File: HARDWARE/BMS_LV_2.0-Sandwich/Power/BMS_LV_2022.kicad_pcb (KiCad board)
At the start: 4 copper layers, 90 x 45 mm, 104 parts, among them J1 Conn_01x26, J11 Conn_01x07_Female, J2 AS214-97PN, J4 Battery+, J5 Battery-, Q1 BC846, Q10 BSS138, Q12 SIR5607DP-T1-RE3, Q13 SIR5607DP-T1-RE3, Q14 SIR5607DP-T1-RE3, Q15 SIR5607DP-T1-RE3, Q2 ZXMN3F30FHTA, Q3 ZXMN3F30FHTA, Q4 ZXMN3F30FHTA, Q5 ZXMN3F30FHTA, Q6 ZXMN3F30FHTA, Q7 ZXMN3F30FHTA, U5 ACHS-7123

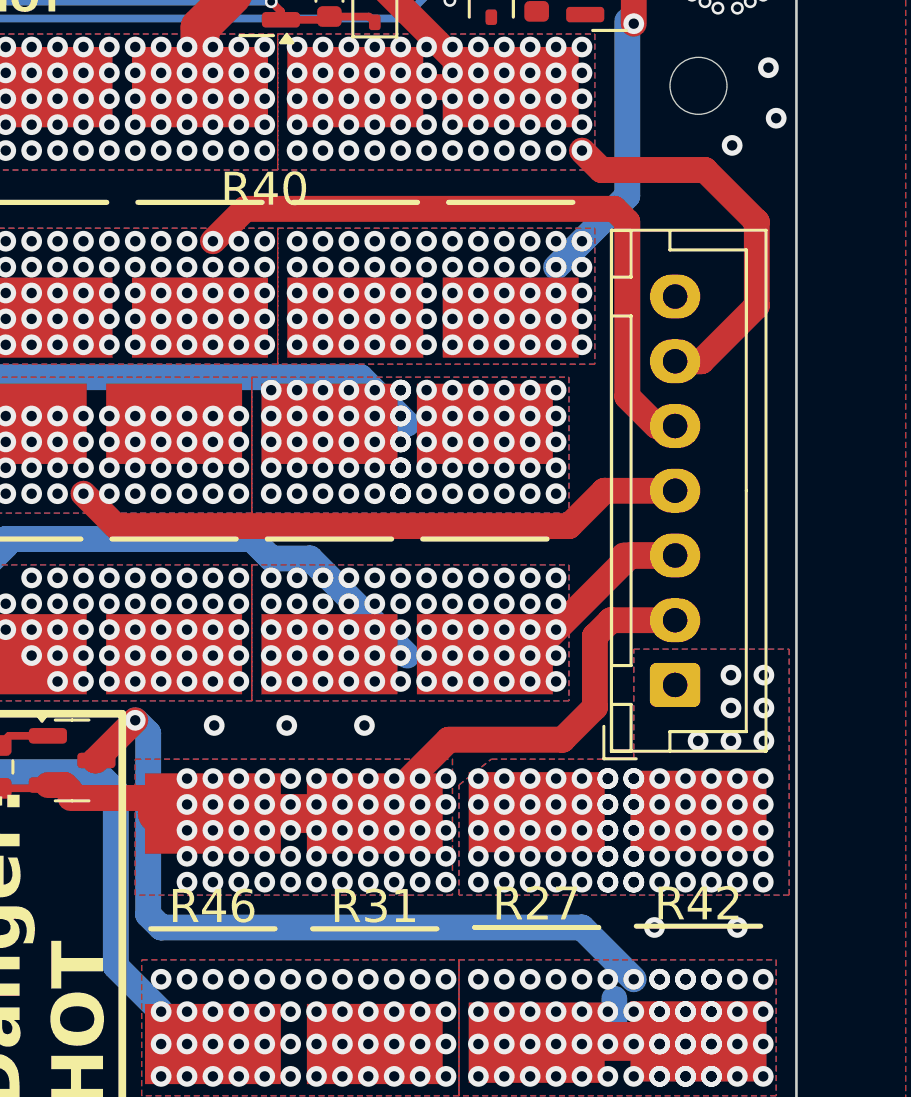
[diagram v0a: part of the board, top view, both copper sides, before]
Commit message: Zmieniono tvs, dodano znowu uart, poprawiono silkscreen, gotowy na release
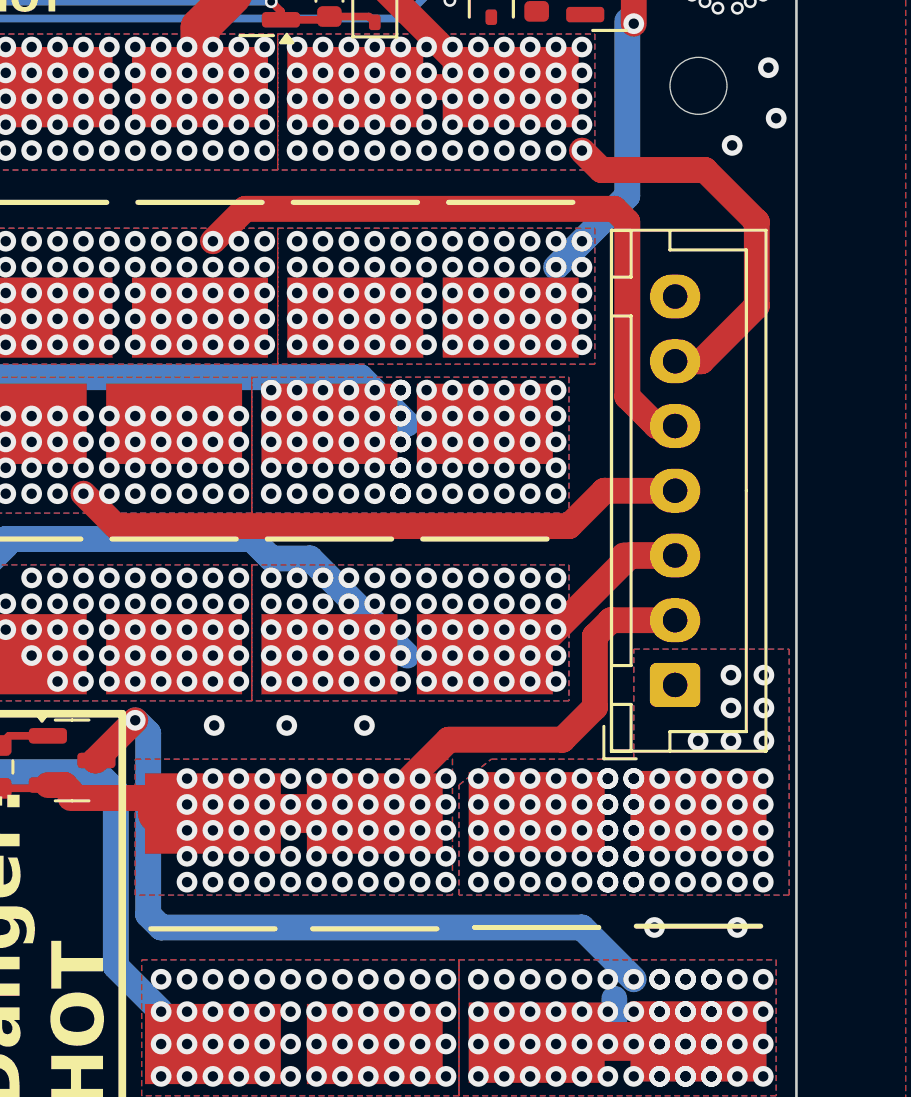
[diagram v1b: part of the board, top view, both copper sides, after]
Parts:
- removed the G*** at (150.0, 101.3)
- added G***: LOGO, footprints:zab2, B.Cu at (147.7, 100.8)
